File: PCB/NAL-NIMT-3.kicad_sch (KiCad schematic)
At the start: 27 parts

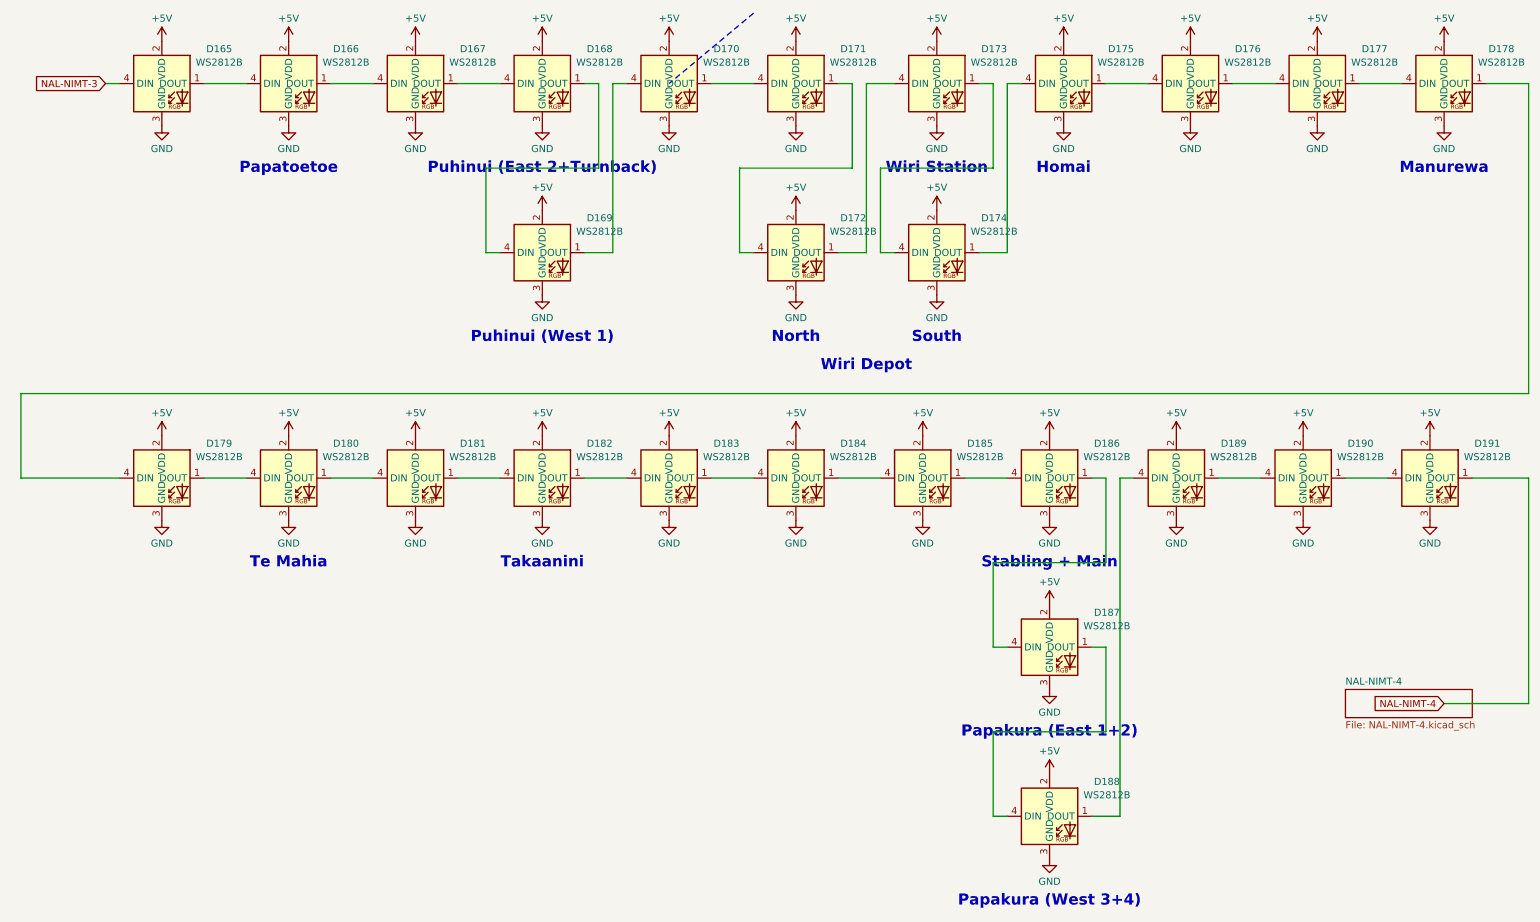
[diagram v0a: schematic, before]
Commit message: Final tweaks for V1.0.0
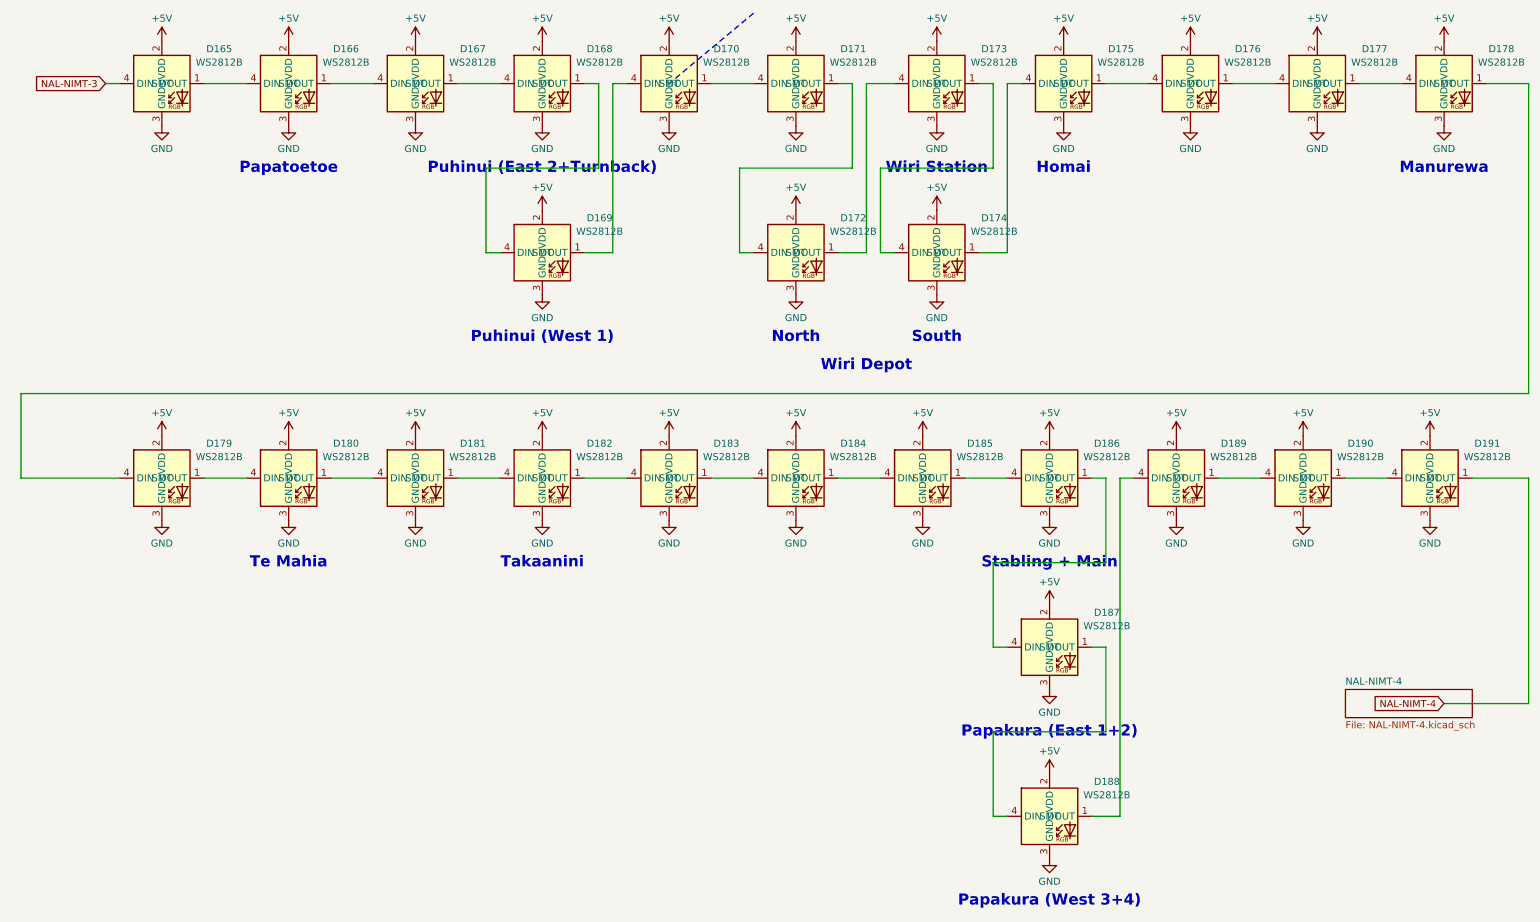
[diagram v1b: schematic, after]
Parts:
- D165, D166, D167, D168, D169, D170, D171, D172, D173, D174, D175, D176, D177, D178, D179, D180, D181, D182, D183, D184, D185, D186, D187, D188, D189, D190, D191: Manufacturer (none) -> XINGLIGHT; Part (none) -> XL-1615RGBC-WS2812B; Process (none) -> SMT
